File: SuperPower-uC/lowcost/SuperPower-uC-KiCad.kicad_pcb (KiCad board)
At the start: 2 copper layers, 83.6 x 28.4 mm, 81 parts, among them J1 Battery connector, J2 Thermistor, J3 USB_B_Micro, J4 Solar in, J5 main pin header fight, J6 main pin header left, Q1 2N7002, Q2 2N7002, Q3 S8050, Q4 S8050, Q5 AO3401A, Q6 AO3401A, Q7 2N7002, U1 FS312F-G, U10 FP6291LR, U11 ME6210A33P, U12 ME6210A33P, U13 ESP32-WROOM32, U2 FS8205A, U3 LC709203FQH, U4 TP4056, U5 CH340G, U6 AMS1117-3.3, U7 PCF8563T, U8 XC6206P332MR, U9 TCA6408A, Y1 12MHZ, Y2 32.768KHz

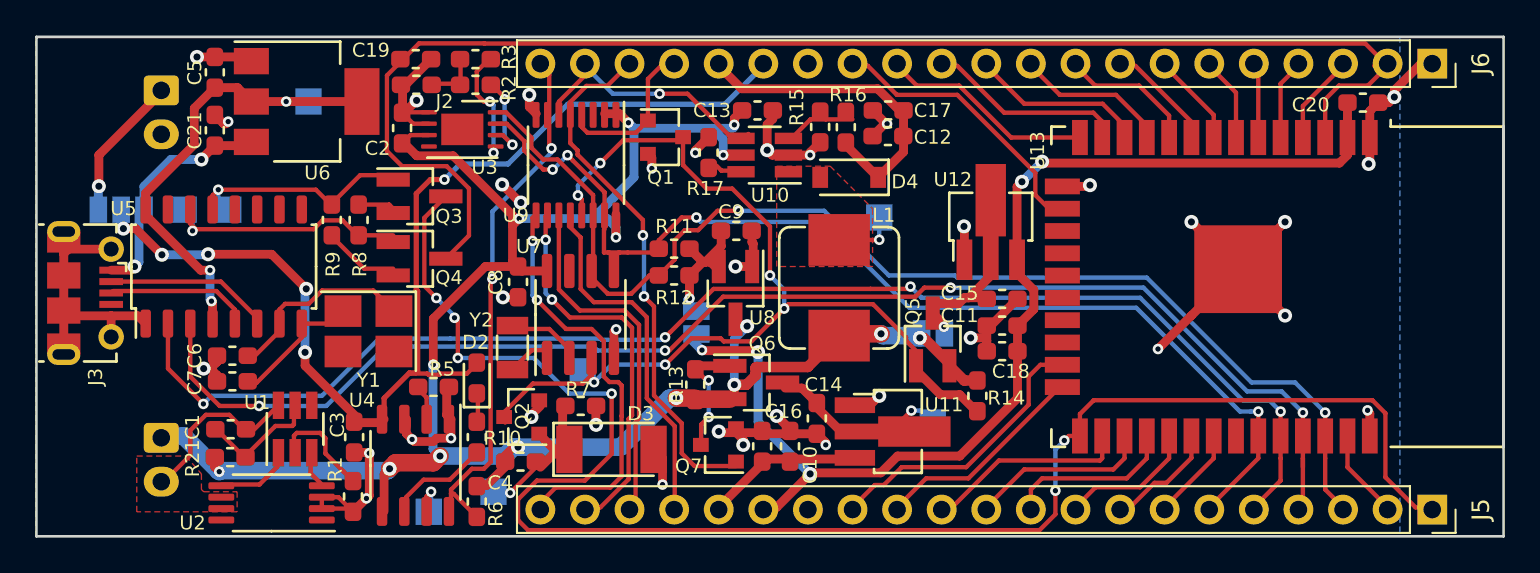
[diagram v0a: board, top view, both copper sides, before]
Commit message: even more optimisation
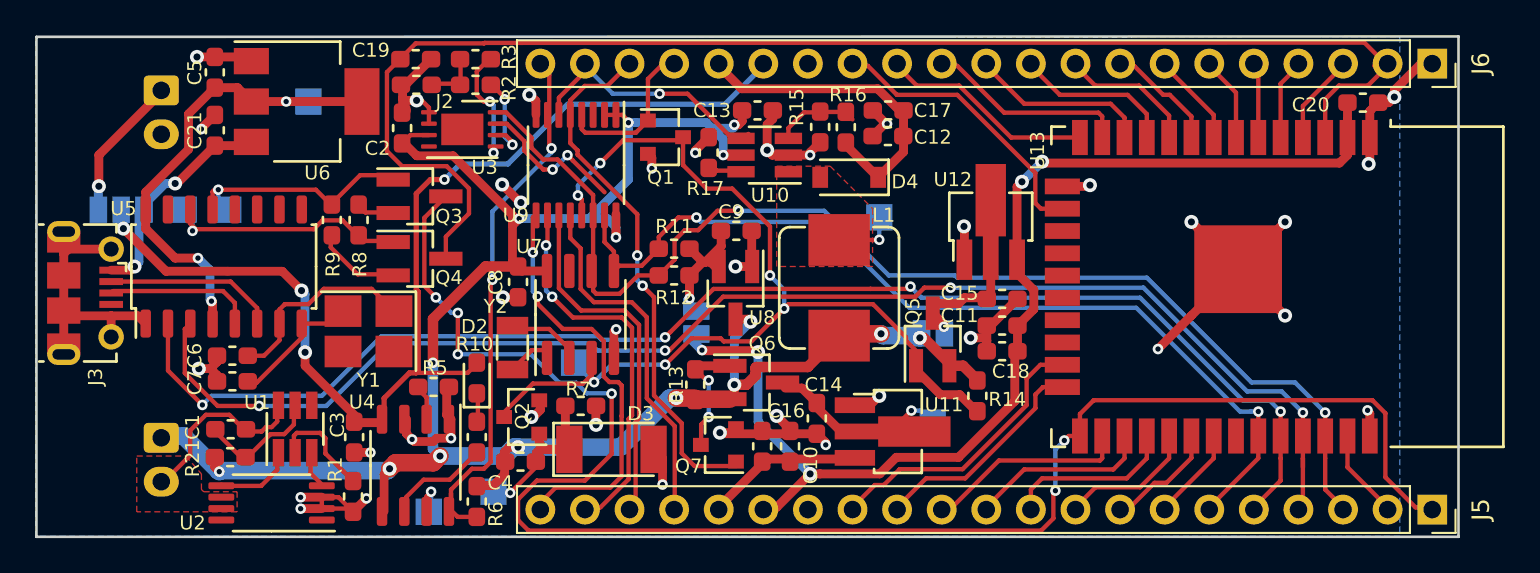
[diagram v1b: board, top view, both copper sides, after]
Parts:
- moved TP2 0.70 mm to (132.6, 113.5)
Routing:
- net /Charging Module/SDA: track 63.0 -> 61.7 mm
- net Net-(R15-Pad1): track 3.56 -> 4.80 mm
- net GND: track 116.4 -> 115.3 mm, vias 37 -> 38
- net /Battery Module/VBAT: track 118.2 -> 119.0 mm
- net /Charger I/O/3v3FTDI: track 26.9 -> 27.7 mm
- net /Charger I/O/VCHARGE: track 64.4 -> 63.8 mm, vias 6 -> 4
- net /Charger I/O/VBUS: track 13.5 -> 12.9 mm
- net Net-(C15-Pad1): track 7.07 -> 6.47 mm
- net CH_DIS: track 30.8 -> 31.3 mm
- net Net-(C1-Pad2): track 9.70 -> 10.2 mm
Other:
- board size 83.6 x 28.4 mm -> 81 x 28.5 mm
